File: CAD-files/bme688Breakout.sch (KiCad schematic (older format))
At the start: 9 parts, among them J1 Castellated_Conn_01x04, U1 BME688

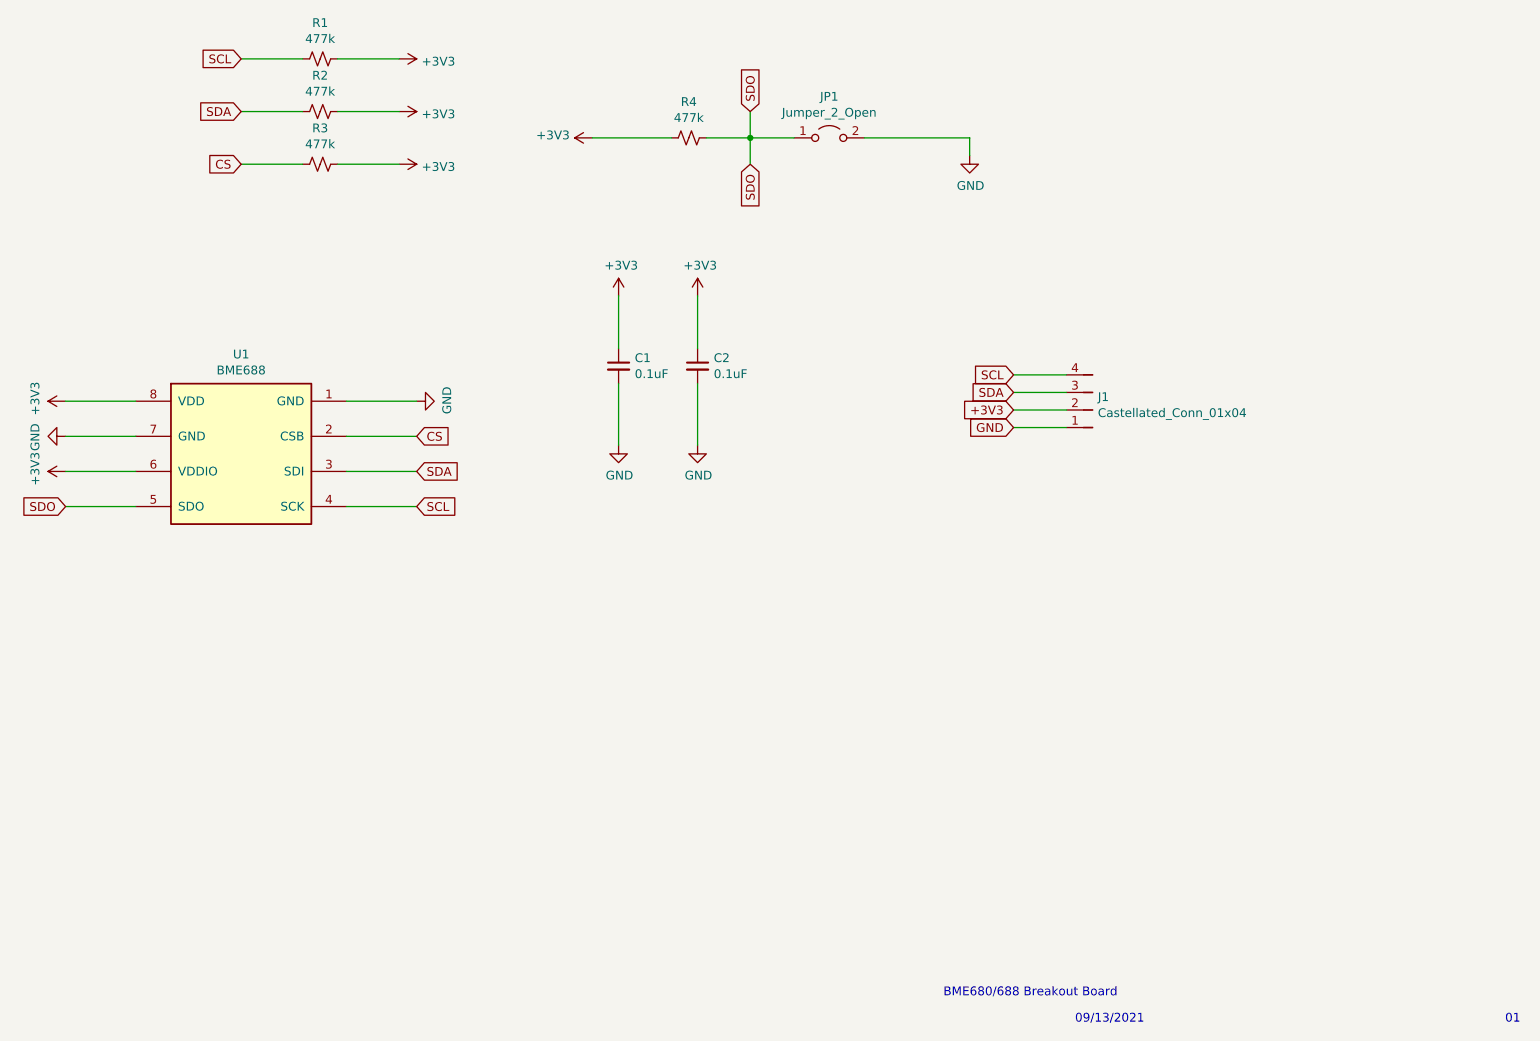
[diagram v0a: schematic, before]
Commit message: Add files via upload
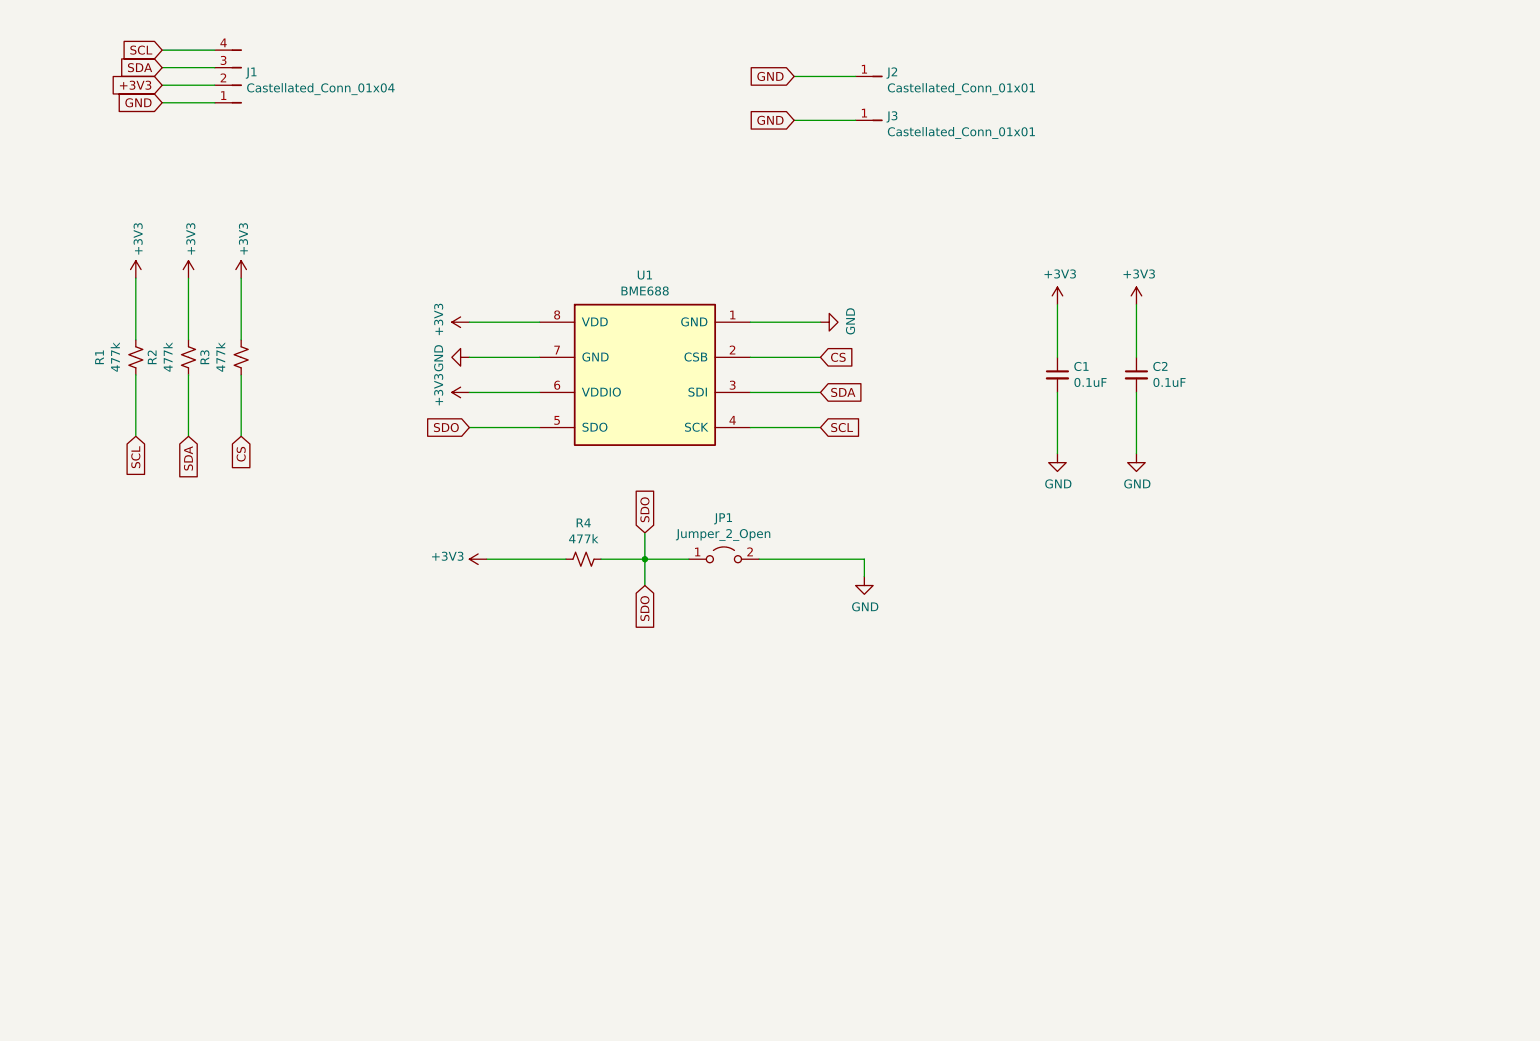
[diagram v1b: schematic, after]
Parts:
- added J2, J3: Castellated_Conn_01x01, DS-connectors:Castellated_PinHeader_01x01_P2.54mm_Vertical, symbol DS-connectors:Castellated_Conn_01x01
- C1, C2: footprint Capacitor_SMD:C_0603_1608Metric -> Capacitor_SMD:C_0805_2012Metric
- R1, R2, R3, R4: footprint Resistor_SMD:R_0603_1608Metric -> Resistor_SMD:R_0805_2012Metric
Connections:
- net GND: now also J2.1, J3.1
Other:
- note removed: "01"
- note removed: "09/13/2021"
- note removed: "BME680/688 Breakout Board"
- moved on the sheet: C1, C2, J1, JP1, R1, R2, R3, R4, U1
